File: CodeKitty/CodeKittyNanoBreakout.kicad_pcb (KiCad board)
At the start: 2 copper layers, 17.8 x 43.2 mm, 14 parts, among them P1 CONN_01X02, P2 CONN_01X02, P3 CONN_01X03, P4 CONN_01X03, P5 CONN_01X03, SW1 SW_PUSH_SMALL_H, SW2 Switch_SPDT_x2, U1 ArduinoNano

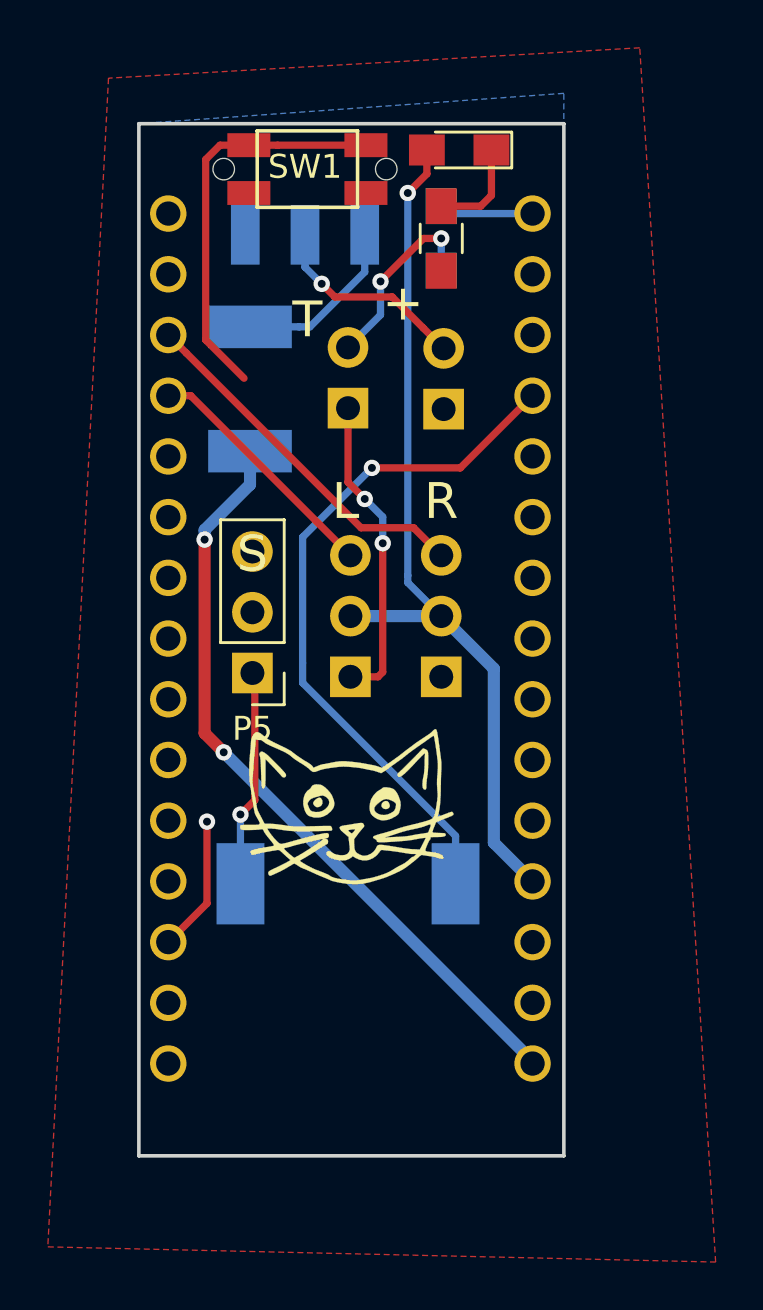
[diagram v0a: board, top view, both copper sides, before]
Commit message: ServoTester first commit
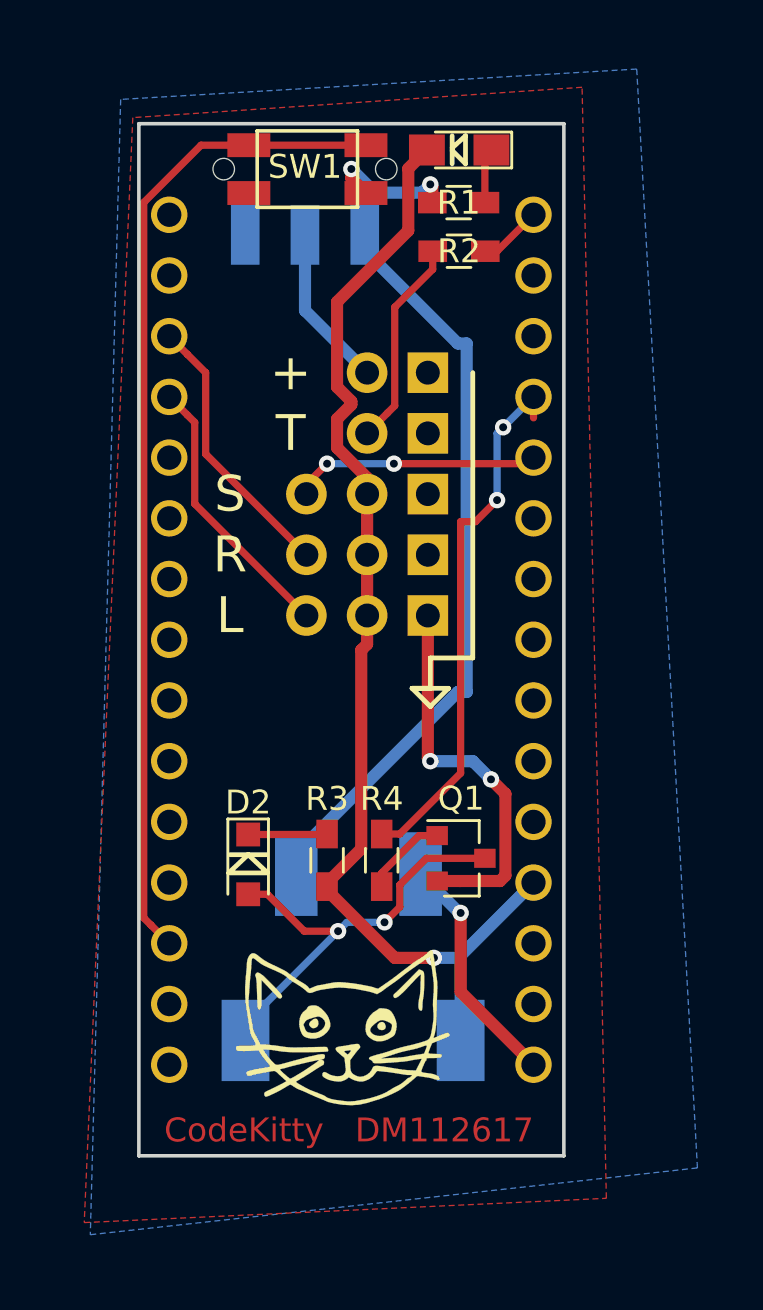
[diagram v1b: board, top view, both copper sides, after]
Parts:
- added D2: D, Diodes_SMD:D_SOD-323_HandSoldering, F.Cu at (201.4, 113.5)
- added Q1: MMBT3904, TO_SOT_Packages_SMD:SOT-23, F.Cu at (210.3, 113.3)
- added R3: R, Resistors_SMD:R_0603_HandSoldering, F.Cu at (204.7, 113.4)
- added R4: R, Resistors_SMD:R_0603_HandSoldering, F.Cu at (207.0, 113.4)
- P5: moved to B.Cu
- R1: footprint Resistors_SMD:R_0805_HandSoldering -> Resistors_SMD:R_0603_HandSoldering
- R2: footprint Resistors_SMD:R_0805_HandSoldering -> Resistors_SMD:R_0603_HandSoldering; moved to F.Cu
- moved F1 20.8 mm to (206.0, 113.9), turned to 180 degrees
- moved P5 10.5 mm to (208.9, 98.0), turned to 90 degrees
- moved G*** 9.25 mm to (205.2, 120.4)
- moved SP1 6.56 mm to (205.8, 120.9)
- moved P4 5.13 mm to (208.9, 100.6), turned to 90 degrees
- moved P3 4.13 mm to (208.9, 103.1), turned to 90 degrees
- moved P2 3.50 mm to (208.9, 95.5), turned to 90 degrees
- moved R1 1.67 mm to (210.2, 85.9), turned to 180 degrees
- moved P1 1.66 mm to (208.9, 93.0), turned to 90 degrees
- moved R2 0.92 mm to (210.2, 87.9), turned to 0 degrees
- moved U1 0.06 mm to (205.7, 104.1)
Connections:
- SP1 pad 1: BUZZ -> 5V
- SP1 pad 2: GND -> Net-(D2-Pad2)
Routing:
- net Net-(F1-Pad1): track 7.31 -> 31.9 mm
- net VCC: track 32.1 -> 9.96 mm, vias 2 -> 1
- net RST: track 22.5 -> 41.7 mm, vias 1 -> 0
- net Net-(D2-Pad2): track 0.00 -> 18.5 mm, vias 0 -> 2
- net 5V: track 36.8 -> 48.9 mm
- net SENS: track 0.00 -> 10.4 mm, vias 0 -> 2
- net BUZZ: track 29.2 -> 22.6 mm, vias 1 -> 2
- net RSERVO: track 15.2 -> 11.5 mm
- net Net-(Q1-Pad1): track 0.00 -> 3.54 mm
- net Net-(D2-Pad1): track 0.00 -> 3.31 mm
- net Net-(D1-Pad1): track 4.19 -> 2.31 mm
- net Net-(P1-Pad2): track 8.56 -> 6.84 mm, vias 1 -> 0
- net TAIL: track 3.95 -> 2.65 mm
- net LSERVO: track 10.4 -> 11.5 mm
- net Net-(P2-Pad2): track 8.66 -> 8.76 mm, vias 2 -> 0
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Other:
- board text added: "CodeKitty DM112617"
- board text removed: "-"
- board text removed: "1"
- board text removed: "BATT"
- board text removed: "CodeKitty DM100917"
- board text removed: "LEFT"
- board text removed: "RIGHT"
- board text removed: "SPKR"
- board text removed: "TAIL"
